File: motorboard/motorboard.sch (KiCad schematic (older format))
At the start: 29 parts, among them J1 Stepper, J2 USB_B, J3 DC Motor, J4 LiPo, J5 UART, J6 Encoders, J7 ICSP, U1 TB6612FNG, U2 ATmega32U4-AU, Y1 8MHz

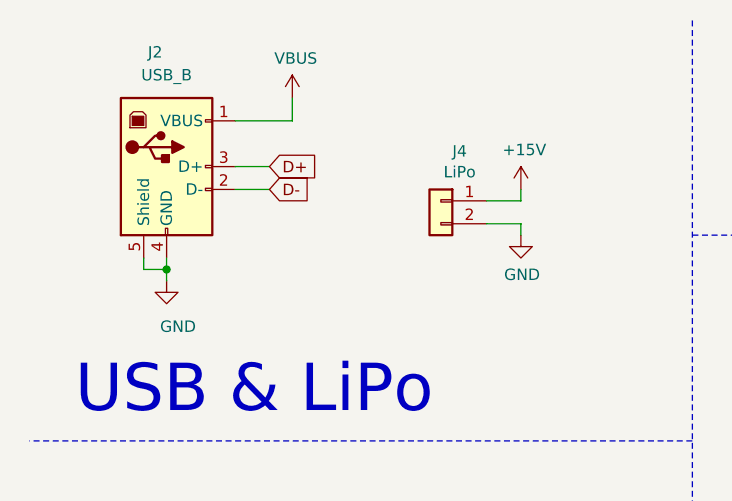
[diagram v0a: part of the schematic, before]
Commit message: GitHub works again!
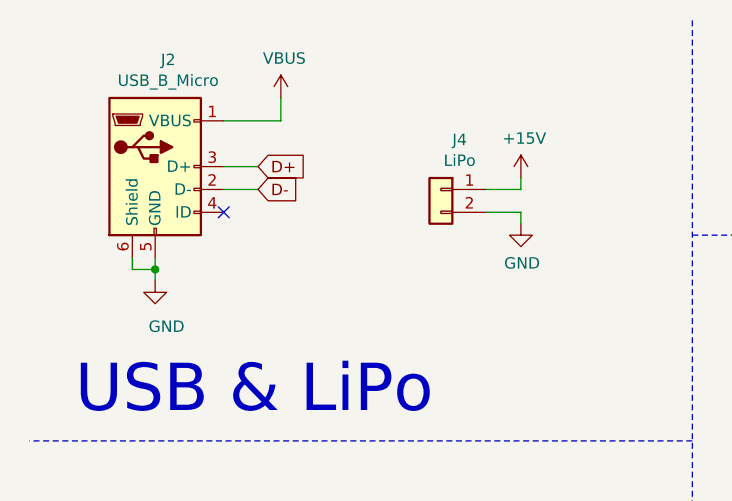
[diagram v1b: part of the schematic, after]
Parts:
- removed J2: USB_B, Connector_USB:USB_B_OST_USB-B1HSxx_Horizontal, symbol Connector:USB_B
- added J2: USB_B_Micro, symbol Connector:USB_B_Micro
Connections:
- net D+: now also J2.3 (D+)
- net D-: now also J2.2 (D-)
- net GND: now also J2.5 (GND), J2.6 (Shield)
- net VBUS: now also J2.1 (VBUS)
- no-connect marks 20 -> 21
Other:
- moved on the sheet: J4
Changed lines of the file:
@@
 $EndComp
 Wire Wire Line
-	1850 1100 1850 1000
-Wire Wire Line
-	1600 1100 1850 1100
-Text GLabel 1750 1400 2    50   Input ~ 0
+	1800 1100 1800 1000
+Wire Wire Line
+	1550 1100 1800 1100
+Text GLabel 1700 1400 2    50   Input ~ 0
 D-
-Text GLabel 1750 1300 2    50   Input ~ 0
+Text GLabel 1700 1300 2    50   Input ~ 0
 D+
 Wire Wire Line
-	1600 1400 1750 1400
-Wire Wire Line
-	1600 1300 1750 1300
-$Comp
-L Connector:USB_B J2
-U 1 1 5E4E1068
-P 1300 1300
-F 0 "J2" H 1250 1800 50  0000 C CNN
-F 1 "USB_B" H 1300 1700 50  0000 C CNN
-F 2 "Connector_USB:USB_B_OST_USB-B1HSxx_Horizontal" H 1450 1250 50  0001 C CNN
-F 3 " ~" H 1450 1250 50  0001 C CNN
-	1    1300 1300
-	1    0    0    -1
-$EndComp
-Connection ~ 1300 1750
-Wire Wire Line
-	1300 1750 1300 1700
-Wire Wire Line
-	1300 1750 1300 1800
-Wire Wire Line
-	1200 1750 1300 1750
-Wire Wire Line
-	1200 1700 1200 1750
+	1550 1400 1700 1400
+Wire Wire Line
+	1550 1300 1700 1300
+Connection ~ 1250 1750
+Wire Wire Line
+	1250 1750 1250 1700
+Wire Wire Line
+	1250 1750 1250 1800
+Wire Wire Line
+	1150 1750 1250 1750
+Wire Wire Line
+	1150 1700 1150 1750
 $Comp
 L power:GND #PWR03
 U 1 1 5E3E5F09
-P 1300 1800
-F 0 "#PWR03" H 1300 1550 50  0001 C CNN
-F 1 "GND" H 1350 1600 50  0000 C CNN
-F 2 "" H 1300 1800 50  0001 C CNN
-F 3 "" H 1300 1800 50  0001 C CNN
-	1    1300 1800
+P 1250 1800
+F 0 "#PWR03" H 1250 1550 50  0001 C CNN
+F 1 "GND" H 1300 1600 50  0000 C CNN
+F 2 "" H 1250 1800 50  0001 C CNN
+F 3 "" H 1250 1800 50  0001 C CNN
+	1    1250 1800
 	1    0    0    -1
 $EndComp
@@
 L power:VBUS #PWR04
 U 1 1 5E61CDDB
-P 1850 1000
-F 0 "#PWR04" H 1850 850 50  0001 C CNN
-F 1 "VBUS" H 1865 1173 50  0000 C CNN
-F 2 "" H 1850 1000 50  0001 C CNN
-F 3 "" H 1850 1000 50  0001 C CNN
-	1    1850 1000
-	1    0    0    -1
-$EndComp
-Wire Wire Line
-	2850 1550 2700 1550
-Wire Wire Line
-	2700 1450 2850 1450
+P 1800 1000
+F 0 "#PWR04" H 1800 850 50  0001 C CNN
+F 1 "VBUS" H 1815 1173 50  0000 C CNN
+F 2 "" H 1800 1000 50  0001 C CNN
+F 3 "" H 1800 1000 50  0001 C CNN
+	1    1800 1000
+	1    0    0    -1
+$EndComp
+Wire Wire Line
+	2850 1500 2700 1500
+Wire Wire Line
+	2700 1400 2850 1400
 $Comp
 L power:GND #PWR?
 U 1 1 5E649C1D
-P 2850 1600
+P 2850 1550
 AR Path="/5DAD2180/5E649C1D" Ref="#PWR?"  Part="1"
 AR Path="/5E649C1D" Ref="#PWR08"  Part="1"
-F 0 "#PWR08" H 2850 1350 50  0001 C CNN
-F 1 "GND" H 2855 1427 50  0000 C CNN
-F 2 "" H 2850 1600 50  0001 C CNN
-F 3 "" H 2850 1600 50  0001 C CNN
-	1    2850 1600
+F 0 "#PWR08" H 2850 1300 50  0001 C CNN
+F 1 "GND" H 2855 1377 50  0000 C CNN
+F 2 "" H 2850 1550 50  0001 C CNN
+F 3 "" H 2850 1550 50  0001 C CNN
+	1    2850 1550
 	1    0    0    -1
 $EndComp
@@
 L Connector_Generic:Conn_01x02 J?
 U 1 1 5E649C23
-P 2500 1450
+P 2500 1400
 AR Path="/5DAD2180/5E649C23" Ref="J?"  Part="1"
 AR Path="/5E649C23" Ref="J4"  Part="1"
-F 0 "J4" H 2418 1667 50  0000 C CNN
-F 1 "LiPo" H 2418 1576 50  0000 C CNN
-F 2 "Connector_PinHeader_2.54mm:PinHeader_1x02_P2.54mm_Vertical" H 2500 1450 50  0001 C CNN
-F 3 "~" H 2500 1450 50  0001 C CNN
-	1    2500 1450
+F 0 "J4" H 2418 1617 50  0000 C CNN
+F 1 "LiPo" H 2418 1526 50  0000 C CNN
+F 2 "Connector_PinHeader_2.54mm:PinHeader_1x02_P2.54mm_Vertical" H 2500 1400 50  0001 C CNN
+F 3 "~" H 2500 1400 50  0001 C CNN
+	1    2500 1400
 	-1   0    0    -1
 $EndComp
 Wire Wire Line
-	2850 1400 2850 1450
-Wire Wire Line
-	2850 1600 2850 1550
+	2850 1350 2850 1400
+Wire Wire Line
+	2850 1550 2850 1500
 $Comp
 L power:+15V #PWR?
 U 1 1 5E649C2B
-P 2850 1400
+P 2850 1350
 AR Path="/5DAD2180/5E649C2B" Ref="#PWR?"  Part="1"
 AR Path="/5E649C2B" Ref="#PWR07"  Part="1"
-F 0 "#PWR07" H 2850 1250 50  0001 C CNN
-F 1 "+15V" H 2865 1573 50  0000 C CNN
-F 2 "" H 2850 1400 50  0001 C CNN
-F 3 "" H 2850 1400 50  0001 C CNN
-	1    2850 1400
+F 0 "#PWR07" H 2850 1200 50  0001 C CNN
+F 1 "+15V" H 2865 1523 50  0000 C CNN
+F 2 "" H 2850 1350 50  0001 C CNN
+F 3 "" H 2850 1350 50  0001 C CNN
+	1    2850 1350
 	1    0    0    -1
 $EndComp
@@
 	1    0    0    -1
 $EndComp
+$Comp
+L Connector:USB_B_Micro J2
+U 1 1 5E58BFE0
+P 1250 1300
+F 0 "J2" H 1307 1767 50  0000 C CNN
+F 1 "USB_B_Micro" H 1307 1676 50  0000 C CNN
+F 2 "" H 1400 1250 50  0001 C CNN
+F 3 "~" H 1400 1250 50  0001 C CNN
+	1    1250 1300
+	1    0    0    -1
+$EndComp
+NoConn ~ 1550 1500
 $EndSCHEMATC
